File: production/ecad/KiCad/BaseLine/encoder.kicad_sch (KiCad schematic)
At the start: 10 parts, among them J5 Rotary Encoder Connector, U9 TXB0104DR

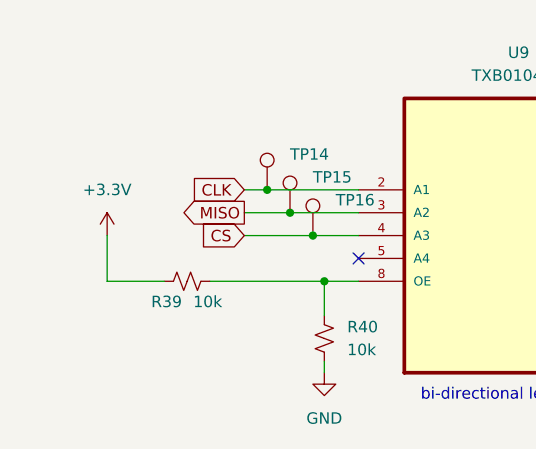
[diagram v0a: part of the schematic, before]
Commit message: rotary enc net names
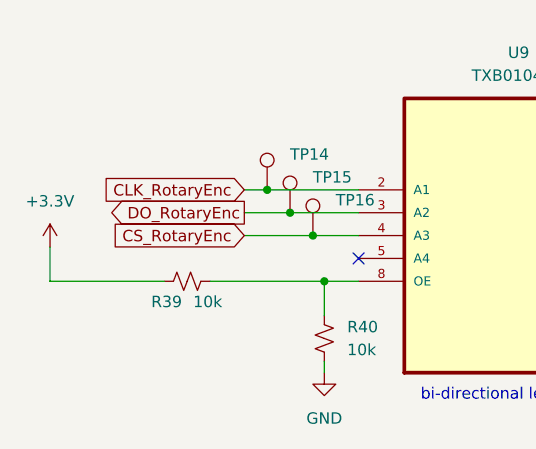
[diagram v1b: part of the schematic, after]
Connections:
- net CLK renamed CLK_RotaryEnc
- net CS renamed CS_RotaryEnc
- net MISO renamed DO_RotaryEnc
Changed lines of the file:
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@@
 	(wire
 		(pts
-			(xy 46.99 71.12) (xy 40.64 71.12)
+			(xy 46.99 71.12) (xy 34.29 71.12)
 		)
 		(stroke
@@
 	(wire
 		(pts
-			(xy 40.64 71.12) (xy 40.64 66.04)
+			(xy 34.29 71.12) (xy 34.29 67.31)
 		)
 		(stroke
@@
 		)
 	)
-	(global_label "MISO"
+	(global_label "DO_RotaryEnc"
 		(shape output)
 		(at 55.88 63.5 180)
@@
 		)
 		(property "Intersheetrefs" "${INTERSHEET_REFS}"
-			(at 48.2986 63.5 0)
+			(at 39.8926 63.5 0)
 			(effects
 				(font
@@
 		)
 	)
-	(global_label "CLK"
+	(global_label "CLK_RotaryEnc"
 		(shape input)
 		(at 55.88 60.96 180)
@@
 		)
 		(property "Intersheetrefs" "${INTERSHEET_REFS}"
-			(at 49.3267 60.96 0)
+			(at 38.925 60.96 0)
 			(effects
 				(font
@@
 		)
 	)
-	(global_label "CS"
+	(global_label "CS_RotaryEnc"
 		(shape input)
 		(at 55.88 66.04 180)
@@
 		)
 		(property "Intersheetrefs" "${INTERSHEET_REFS}"
-			(at 50.4153 66.04 0)
+			(at 40.0136 66.04 0)
 			(effects
 				(font
@@
 	(symbol
 		(lib_id "power:+3.3V")
-		(at 40.64 66.04 0)
+		(at 34.29 67.31 0)
 		(unit 1)
 		(exclude_from_sim no)
@@
 		(fields_autoplaced yes)
 		(property "Reference" "#PWR062"
-			(at 40.64 69.85 0)
+			(at 34.29 71.12 0)
 			(effects
 				(font
@@
 		)
 		(property "Value" "+3.3V"
-			(at 40.64 60.96 0)
+			(at 34.29 62.23 0)
 			(effects
 				(font
@@
 		)
 		(property "Footprint" ""
-			(at 40.64 66.04 0)
+			(at 34.29 67.31 0)
 			(effects
 				(font
@@
 		)
 		(property "Datasheet" ""
-			(at 40.64 66.04 0)
+			(at 34.29 67.31 0)
 			(effects
 				(font
@@
 		)
 		(property "Description" "Power symbol creates a global label with name \"+3.3V\""
-			(at 40.64 66.04 0)
-			(effects
-				(font
+			(at 34.29 67.31 0)
+			(effects
+				(font

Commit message: Rohi changes
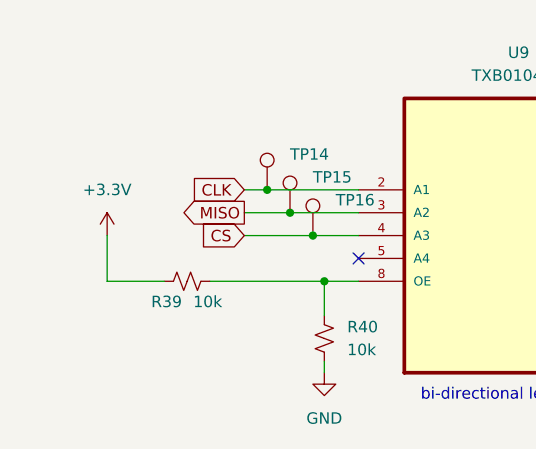
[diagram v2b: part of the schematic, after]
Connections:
- net CLK_RotaryEnc renamed CLK
- net CS_RotaryEnc renamed CS
- net DO_RotaryEnc renamed MISO
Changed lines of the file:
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@@
 	(wire
 		(pts
-			(xy 46.99 71.12) (xy 34.29 71.12)
+			(xy 46.99 71.12) (xy 40.64 71.12)
 		)
 		(stroke
@@
 	(wire
 		(pts
-			(xy 34.29 71.12) (xy 34.29 67.31)
+			(xy 40.64 71.12) (xy 40.64 66.04)
 		)
 		(stroke
@@
 		)
 	)
-	(global_label "DO_RotaryEnc"
+	(global_label "MISO"
 		(shape output)
 		(at 55.88 63.5 180)
@@
 		)
 		(property "Intersheetrefs" "${INTERSHEET_REFS}"
-			(at 39.8926 63.5 0)
+			(at 48.2986 63.5 0)
 			(effects
 				(font
@@
 		)
 	)
-	(global_label "CLK_RotaryEnc"
+	(global_label "CLK"
 		(shape input)
 		(at 55.88 60.96 180)
@@
 		)
 		(property "Intersheetrefs" "${INTERSHEET_REFS}"
-			(at 38.925 60.96 0)
+			(at 49.3267 60.96 0)
 			(effects
 				(font
@@
 		)
 	)
-	(global_label "CS_RotaryEnc"
+	(global_label "CS"
 		(shape input)
 		(at 55.88 66.04 180)
@@
 		)
 		(property "Intersheetrefs" "${INTERSHEET_REFS}"
-			(at 40.0136 66.04 0)
+			(at 50.4153 66.04 0)
 			(effects
 				(font
@@
 	(symbol
 		(lib_id "power:+3.3V")
-		(at 34.29 67.31 0)
+		(at 40.64 66.04 0)
 		(unit 1)
 		(exclude_from_sim no)
@@
 		(fields_autoplaced yes)
 		(property "Reference" "#PWR062"
-			(at 34.29 71.12 0)
+			(at 40.64 69.85 0)
 			(effects
 				(font
@@
 		)
 		(property "Value" "+3.3V"
-			(at 34.29 62.23 0)
+			(at 40.64 60.96 0)
 			(effects
 				(font
@@
 		)
 		(property "Footprint" ""
-			(at 34.29 67.31 0)
+			(at 40.64 66.04 0)
 			(effects
 				(font
@@
 		)
 		(property "Datasheet" ""
-			(at 34.29 67.31 0)
+			(at 40.64 66.04 0)
 			(effects
 				(font
@@
 		)
 		(property "Description" "Power symbol creates a global label with name \"+3.3V\""
-			(at 34.29 67.31 0)
-			(effects
-				(font
+			(at 40.64 66.04 0)
+			(effects
+				(font

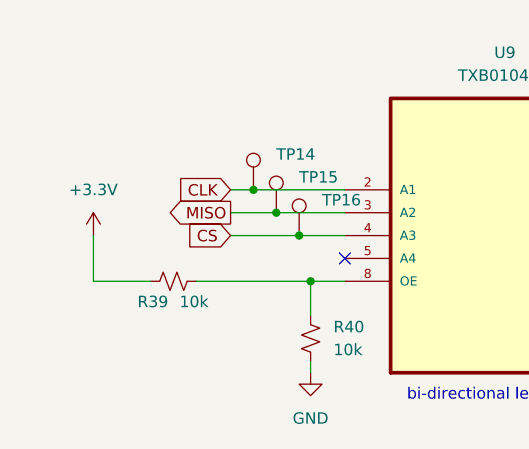
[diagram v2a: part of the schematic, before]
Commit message: if this doesn't work Im killing somebody
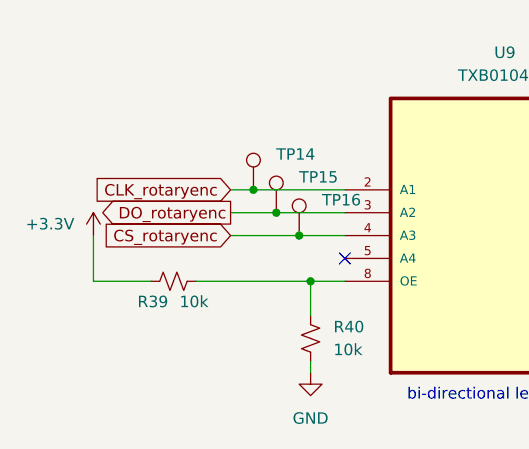
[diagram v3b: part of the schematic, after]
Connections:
- net CLK renamed CLK_rotaryenc
- net CS renamed CS_rotaryenc
- net MISO renamed DO_rotaryenc
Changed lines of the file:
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@@
 		)
 	)
-	(global_label "MISO"
+	(global_label "DO_rotaryenc"
 		(shape output)
 		(at 55.88 63.5 180)
@@
 		)
 		(property "Intersheetrefs" "${INTERSHEET_REFS}"
-			(at 48.2986 63.5 0)
+			(at 40.4368 63.5 0)
 			(effects
 				(font
@@
 		)
 	)
-	(global_label "CLK"
+	(global_label "CLK_rotaryenc"
 		(shape input)
 		(at 55.88 60.96 180)
@@
 		)
 		(property "Intersheetrefs" "${INTERSHEET_REFS}"
-			(at 49.3267 60.96 0)
+			(at 39.4692 60.96 0)
 			(effects
 				(font
@@
 		)
 	)
-	(global_label "CS"
+	(global_label "CS_rotaryenc"
 		(shape input)
 		(at 55.88 66.04 180)
@@
 		)
 		(property "Intersheetrefs" "${INTERSHEET_REFS}"
-			(at 50.4153 66.04 0)
+			(at 40.5578 66.04 0)
 			(effects
 				(font
@@
 		(on_board yes)
 		(dnp no)
-		(fields_autoplaced yes)
 		(property "Reference" "#PWR062"
 			(at 40.64 69.85 0)
@@
 		)
 		(property "Value" "+3.3V"
-			(at 40.64 60.96 0)
-			(effects
-				(font
+			(at 35.814 64.77 0)
+			(effects
+				(font
